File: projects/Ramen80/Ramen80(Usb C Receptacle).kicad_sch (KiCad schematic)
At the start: 5 parts, among them J2 USB_C_RECEPTACLE

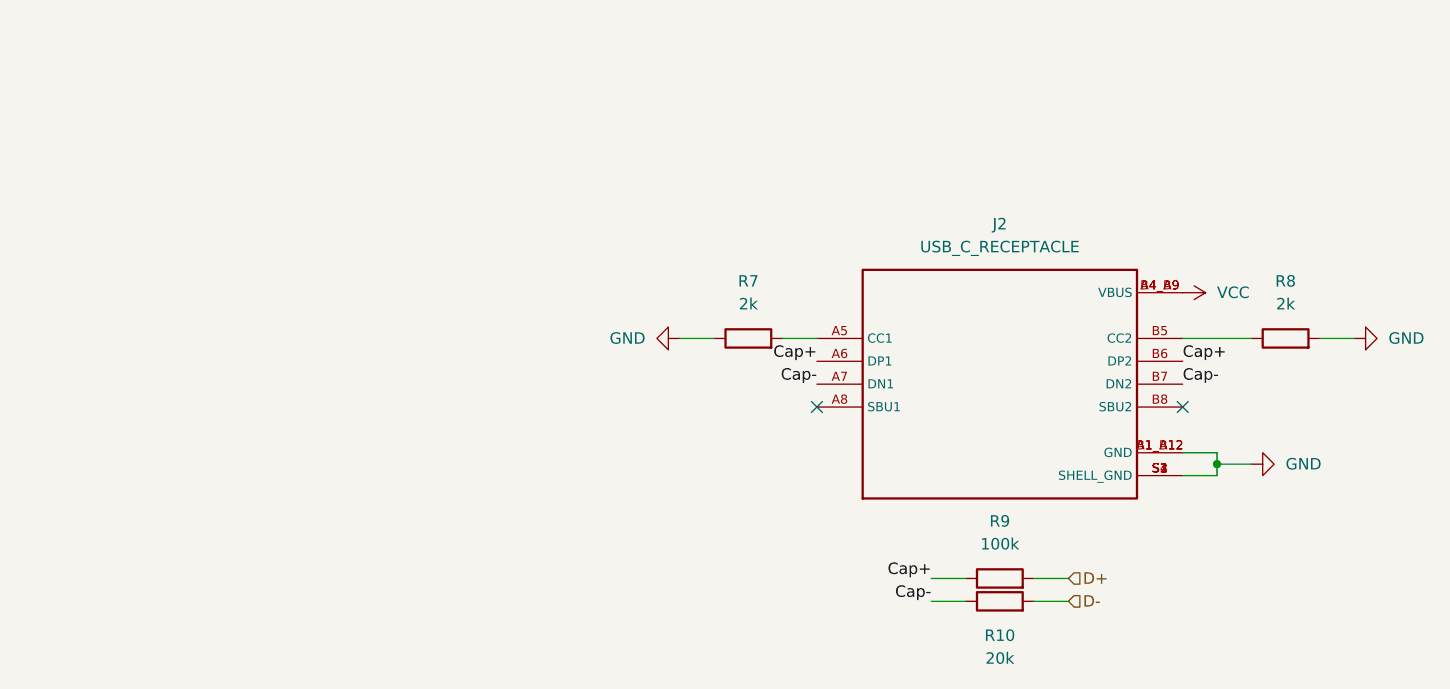
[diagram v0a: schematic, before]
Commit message: Finished PCB
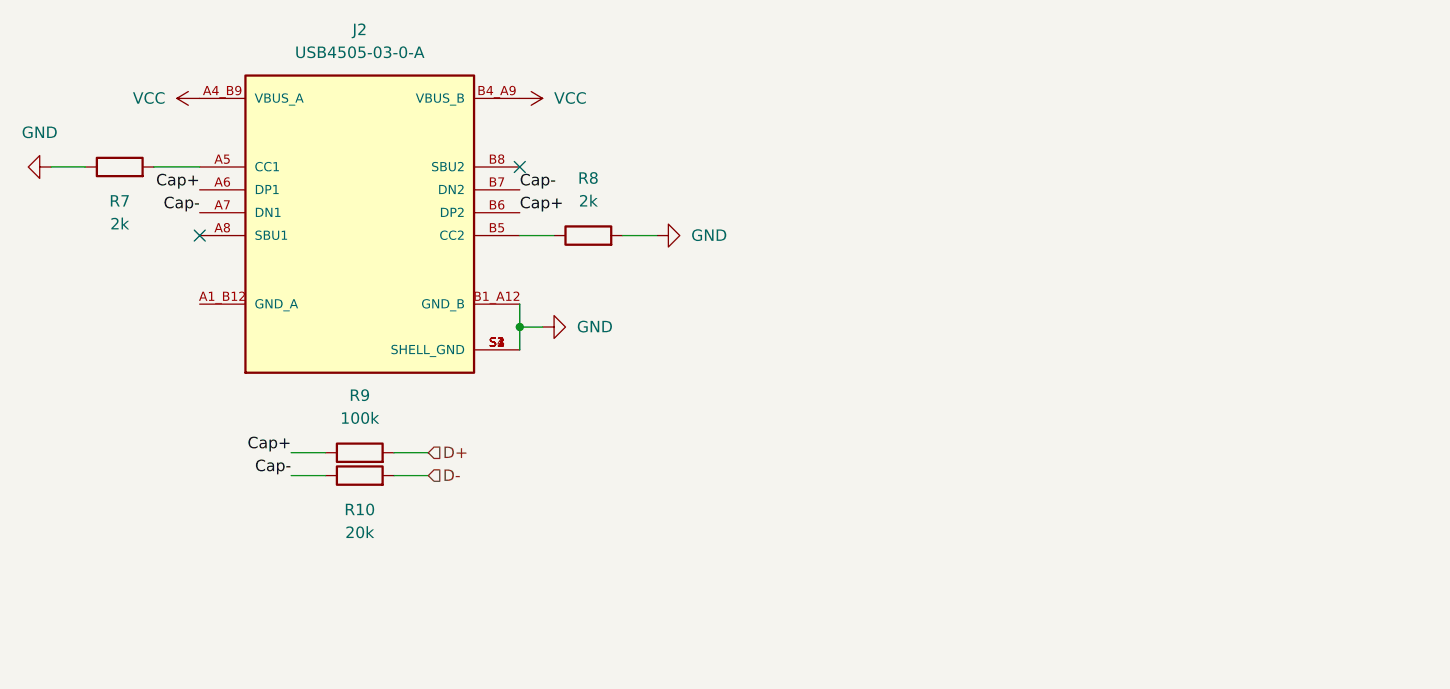
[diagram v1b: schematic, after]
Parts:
- removed J2: USB_C_RECEPTACLE, SamacSys_Parts:GCT_USB4105-GF-A, symbol RamenKeebs:USB4105-GF-A
- added J2: USB4505-03-0-A, RamenKeebs:USB4505-03-0-A, symbol RamenKeebs:USB4505-03-0-A
- R10, R7, R8, R9: footprint Resistor_SMD:R_0805_2012Metric -> RamenKeebs:R_0805
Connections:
- net Cap+: now also J2.A6 (DP1), J2.B6 (DP2)
- net Cap-: now also J2.A7 (DN1), J2.B7 (DN2)
- net GND: now also J2.B1_A12 (GND_B), J2.S1 (SHELL_GND), J2.S2 (SHELL_GND), J2.S3 (SHELL_GND), J2.S4 (SHELL_GND)
- net VCC: now also J2.A4_B9 (VBUS_A), J2.B4_A9 (VBUS_B)
- net at R8.1: now also J2.B5 (CC2)
- net at R7.2: now also J2.A5 (CC1)
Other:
- moved on the sheet: R10, R9
